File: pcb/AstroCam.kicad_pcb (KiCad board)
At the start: 2 copper layers, 40 x 40 mm, 183 parts, among them P1 CONN_01X02, P10 OUTP, P11 CONN_01X01, P12 CONN_01X01, P13 CONN_01X06, P14 LEDS, P15 ADJ, P16 CONN_01X02, P2 CONN_01X18, P3 CONN_01X18, P4 HORI, P5 OUTP, P6 POWER, P7 VERT, P8 CONN_01X06, P9 CONN_01X02, Q1 2SC5095, Q2 MT3S20TU, Q3 2SC5095, Q4 MT3S20TU, Q5 VEC2611, Q6 VEC2607, T1 NET-TIE, T2 NET-TIE, T3 NET-TIE, U1 TPS2420, U11 TPS65530, U12 SN74LVC8T245, U2 LT3487, U3 TPS63002, U4 ADDI7013, U5 ADDI9023, U6 ADA4800, U7 TPS56x200, U8 LMZ10500, U9 ADA4800

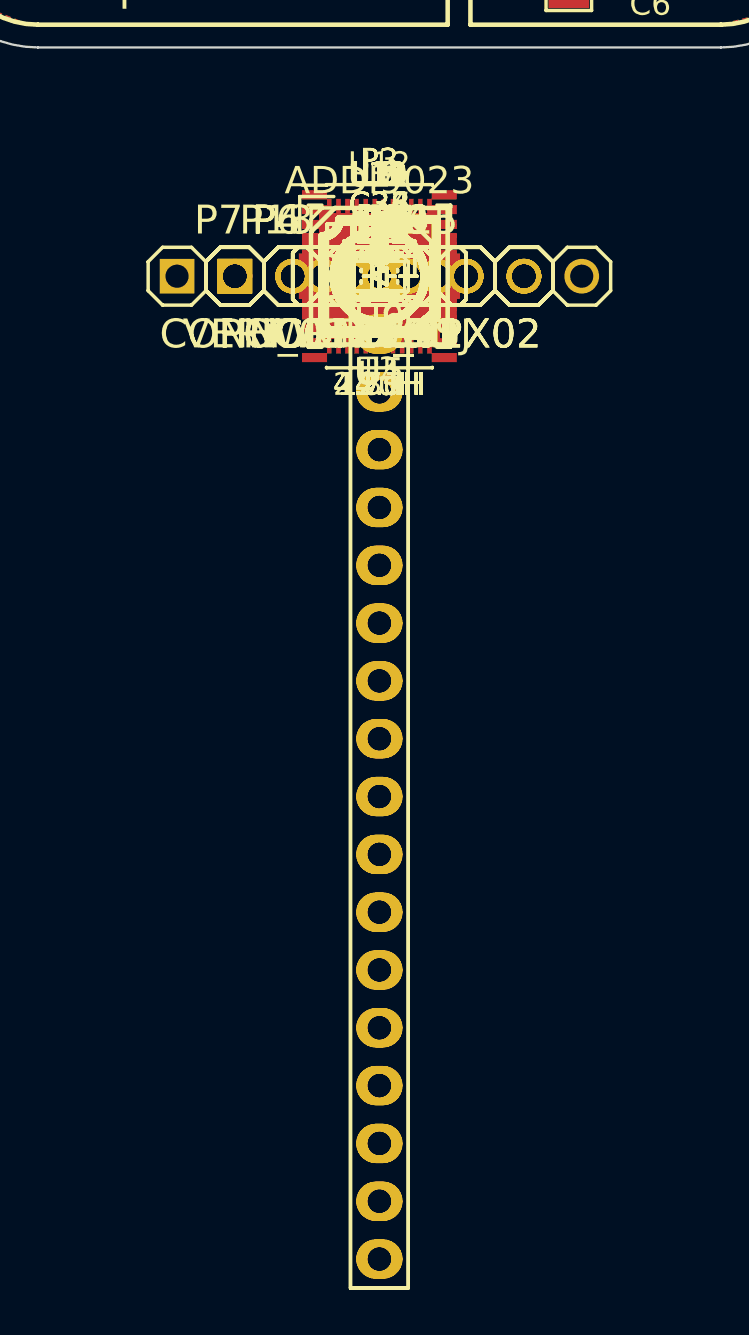
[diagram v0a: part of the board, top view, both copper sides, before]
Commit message: More.
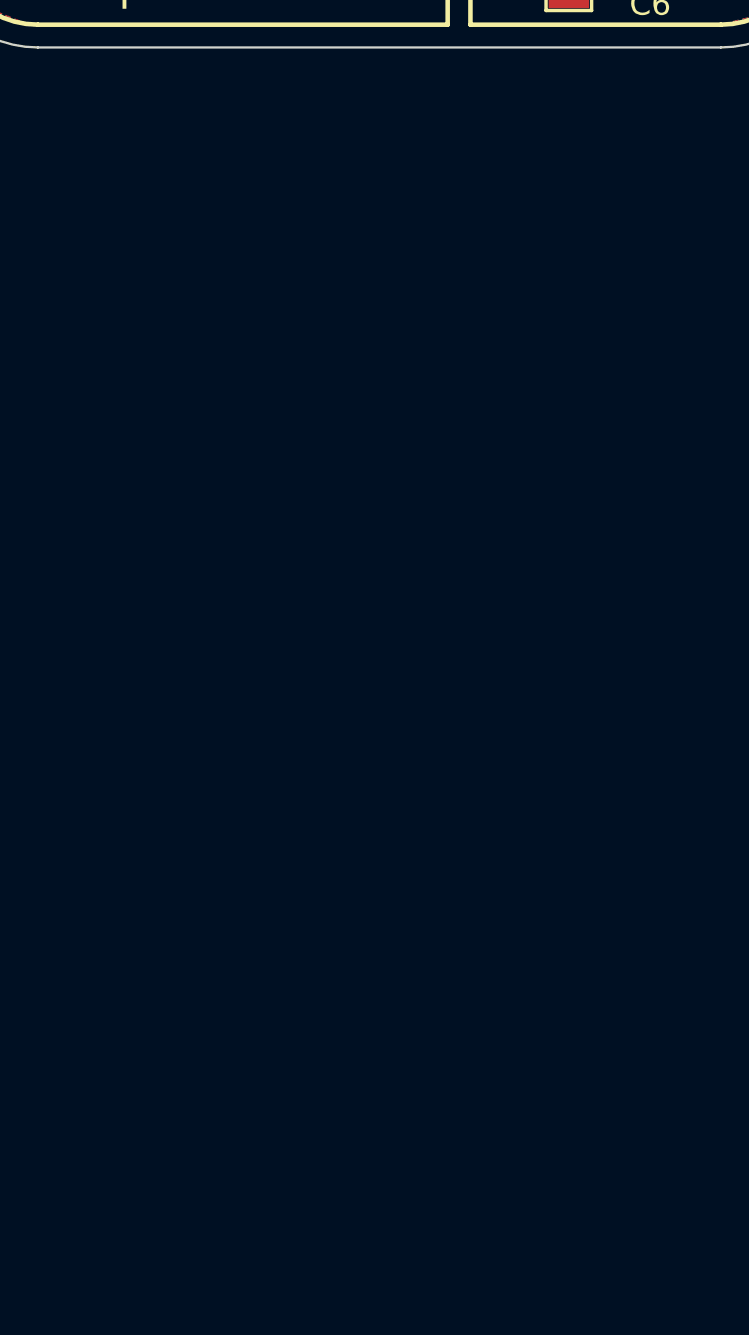
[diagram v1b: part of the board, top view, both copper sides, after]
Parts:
- removed C12, C13, C48, C49: 0.1u, Capacitors_SMD:C_0603_HandSoldering
- removed C17, C38, C39, C40, C41, C42, C43, C44, C45, C46: 0.1uF, Capacitors_SMD:C_0603_HandSoldering
- removed C18: 0.1uF/25V, Capacitors_SMD:C_0603_HandSoldering
- removed C19: 0.1uF/10V, Capacitors_SMD:C_0603_HandSoldering
- removed C22: 1.0uF/25V, Capacitors_SMD:C_0603_HandSoldering
- removed C23: 4.7uF/10V, Capacitors_SMD:c_elec_4x5.3
- removed C24, C26, C27, C29, C50, C51, C52: 0.1uF, Capacitors_SMD:C_0603
- removed C28: 1u/35V, Capacitors_SMD:c_elec_4x5.3
- removed C30: 2200pF, Capacitors_SMD:C_0603
- removed C31, C32: 0.1, Capacitors_SMD:C_0603
- removed C34, C36, C37: 3.3/20V, Capacitors_SMD:c_elec_4x5.3
- removed C35: 0.01, Capacitors_SMD:C_0805_HandSoldering
- removed C47: 4.7uF, Capacitors_SMD:C_0603_HandSoldering
- removed C53, C54: 47uF, Capacitors_Tantalum_SMD:TantalC_SizeA_EIA-3216_Reflow
- removed C55, C56, C58, C72, C75: 10uF, Capacitors_SMD:C_1206
- removed C57: 1.0u, Capacitors_SMD:C_0603
- removed C59: 10u, Capacitors_SMD:C_1206
- removed C60: 3.3uF, Capacitors_SMD:C_0805
- removed C61: 4.7u, Capacitors_SMD:C_0805
- removed C62, C65: 10.0u, Capacitors_SMD:C_1206
- removed C63, C64: 0.1u, Capacitors_SMD:C_0603
- removed C66, C67: 47.0u, Capacitors_SMD:C_1206
- removed C68, C69, C70, C71: 22u, Capacitors_SMD:C_1206
- removed C73, C74: 22uF, Capacitors_SMD:C_1206
- removed C76: 10uF, Capacitors_SMD:C_0805
- removed D2: D, Diodes_SMD:SOD-123
- removed D3, D5: 30V/0.5A, Diodes_SMD:SOD-123
- removed D4: 30V/.5A, Diodes_SMD:SOD-123
- removed JP1, JP2, JP3, JP4: JUMPER3, xess:xess-JP2
- removed L10, L9: 4.7, w_smd_inductors:inductor_smd_4.8x2.8mm
- removed L11: 4.7uH, w_smd_inductors:inductor_smd_4.8x2.8mm
- removed L12: 2.7uH, w_smd_inductors:inductor_smd_4.8x2.8mm
- removed L13, L6, L7: 12uH, w_smd_inductors:inductor_smd_4.8x2.8mm
- removed L5: 4.3uH, w_smd_inductors:inductor_smd_4.8x2.8mm
- removed P1, P16: CONN_01X02, xess:HDR_1x2
- removed P10, P5: OUTP, xess:HDR_1x2
- removed P13: CONN_01X06, xess:HDR_1x6
- removed P14: LEDS, xess:HDR_1x2
- removed P15: ADJ, xess:HDR_1x1
- removed P2, P3: CONN_01X18, Pin_Headers:Pin_Header_Straight_1x18
- removed P4: HORI, xess:HDR_1x6
- removed P6: POWER, xess:HDR_1x6
- removed P7: VERT, xess:HDR_1x8
- removed Q1, Q3: 2SC5095, w_smd_trans:sot323
- removed Q2, Q4: MT3S20TU, w_smd_trans:sot323
- removed Q5: VEC2611, w_smd_trans:sc70
- removed Q6: VEC2607, w_smd_trans:sc70
- removed R10, R11, R14, R15: 10K, Resistors_SMD:R_0603_HandSoldering
- removed R12, R20: 1.17K, Resistors_SMD:R_0603_HandSoldering
- removed R13, R21: 1.74K, Resistors_SMD:R_0603_HandSoldering
- removed R18: 100k, Resistors_SMD:R_0603_HandSoldering
- removed R19: 1M0, Resistors_SMD:R_0603_HandSoldering
- removed R22, R23, R28: 10.0k, Resistors_SMD:R_0603_HandSoldering
- removed R24, R27: 249k, Resistors_SMD:R_0603
- removed R25, R26: 10K, Resistors_SMD:R_0603
- removed R29: 11.0k, Resistors_SMD:R_0603
- removed R30, R40, R42: 5.6k, Resistors_SMD:R_0603
- removed R31, R32, R37, R39, R41, R43, R44, R45, R48: 1.0k, Resistors_SMD:R_0603
- removed R33: 3.0k, Resistors_SMD:R_0603
- removed R34, R35, R36: 0.6k, Resistors_SMD:R_0603
- removed R38: 2.0k, Resistors_SMD:R_0603
- removed R46: 10, Resistors_SMD:R_0603
- removed R47: 5.0k, Resistors_SMD:R_0603
- removed T3: NET-TIE, Oddities:NetTie-I_Connected_SMD
- removed U11: TPS65530, Housings_DFN_QFN:UQFN-48-1EP_6x6mm_Pitch0.4mm
- removed U12: SN74LVC8T245, Housings_SSOP:TSSOP-24_4.4x7.8mm_Pitch0.65mm
- removed U4: ADDI7013, engstad:csp-bga-bc-76-3
- removed U5: ADDI9023, engstad:csp-bga-bc-40-1
- removed U6, U9: ADA4800, engstad:lfcsp-cp-6-4
